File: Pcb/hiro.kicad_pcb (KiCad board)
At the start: 2 copper layers, 80.1 x 107.1 mm, 0 parts

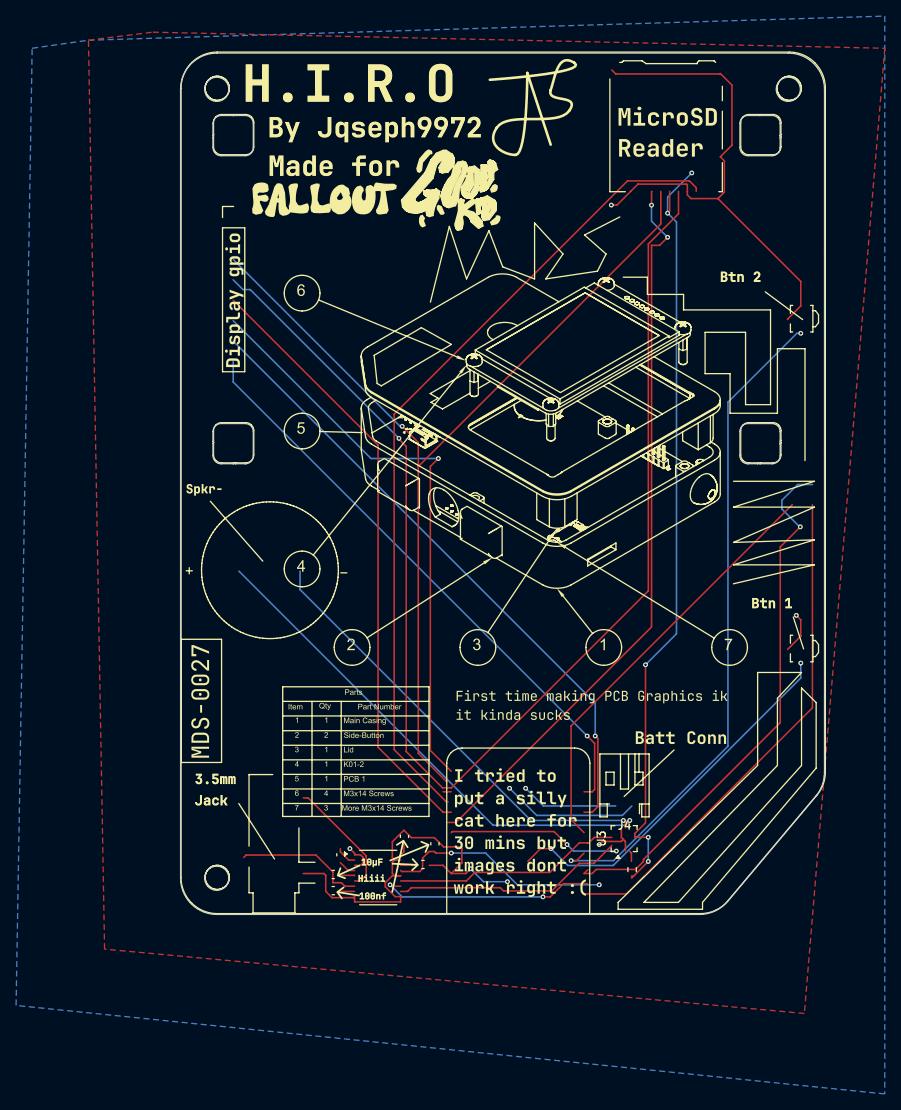
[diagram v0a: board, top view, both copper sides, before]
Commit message: Uh final stuffs i bought emm yayyyy
idk how that pic got there i was sending to my friend idk
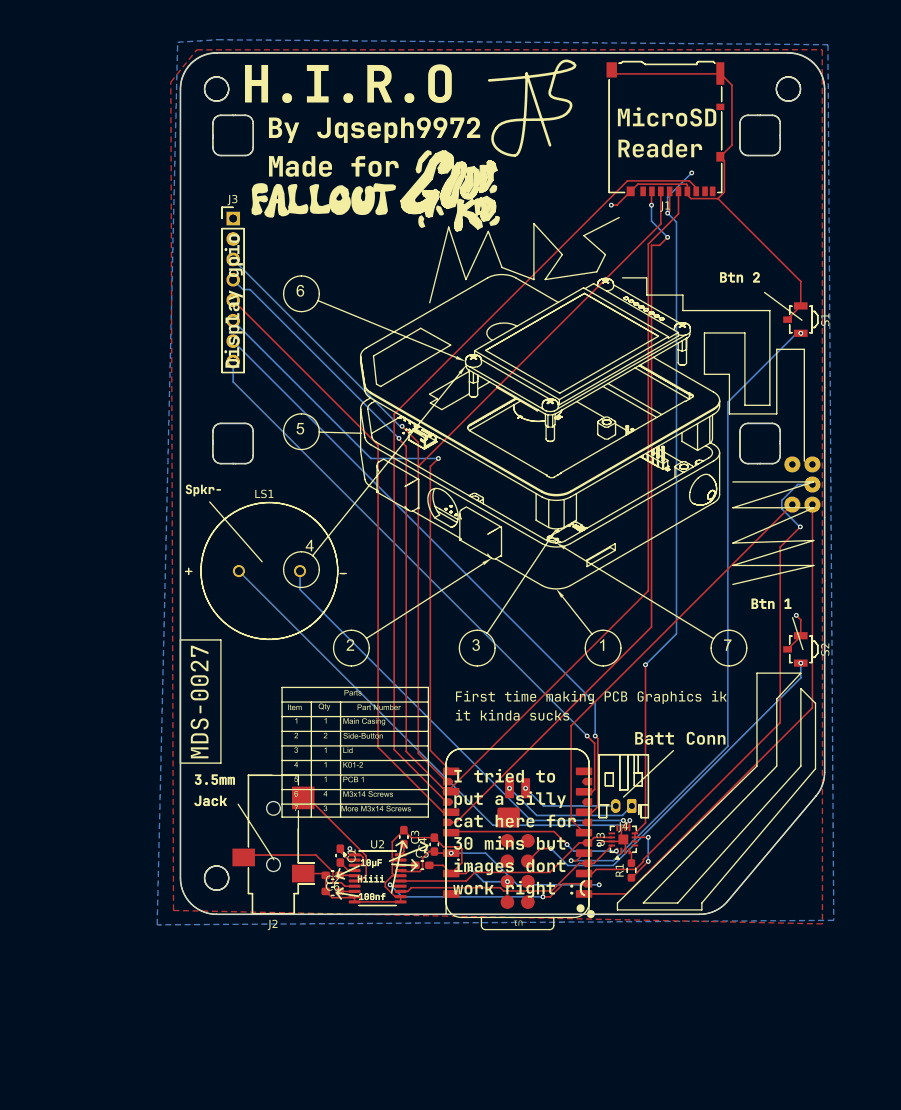
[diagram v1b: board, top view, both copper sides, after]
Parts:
- added C1: 10 µF, Capacitor_SMD:C_0603_1608Metric_Pad1.08x0.95mm_HandSolder, F.Cu at (110.3, 135.4)
- added C2: 100nF, Capacitor_SMD:C_0603_1608Metric_Pad1.08x0.95mm_HandSolder, F.Cu at (109.4, 139.8)
- added C3: 100nF, Capacitor_SMD:C_0603_1608Metric_Pad1.08x0.95mm_HandSolder, F.Cu at (118.2, 133.1)
- added C4: 10 µF, Capacitor_SMD:C_0603_1608Metric_Pad1.08x0.95mm_HandSolder, F.Cu at (122.0, 134.0)
- added C5: 10 µF, Capacitor_SMD:C_0603_1608Metric_Pad1.08x0.95mm_HandSolder, F.Cu at (120.5, 136.6)
- added C6: 10 µF, Capacitor_SMD:C_0603_1608Metric_Pad1.08x0.95mm_HandSolder, F.Cu at (109.4, 137.8)
- added J1: Micro_SD_Card_Det_Hirose_DM3AT, Connector_Card:microSD_HC_Hirose_DM3AT-SF-PEJM5, F.Cu at (150.7, 45.1)
- added J2: AudioJack3, Connector_Audio:Jack_3.5mm_CUI_SJ-3523-SMT_Horizontal, F.Cu at (102.0, 134.0)
- added J3: Conn_01x08, Connector_PinHeader_2.54mm:PinHeader_1x08_P2.54mm_Vertical, F.Cu at (97.0, 56.2)
- added J4: Conn_01x02, Connector_JST:JST_PH_S2B-PH-K_1x02_P2.00mm_Horizontal, F.Cu at (146.6, 129.2)
- added LS1: CVS-1708, Spkr:SPKR_CVS-1708, F.Cu at (101.5, 100.0)
- added R1: 1M, Resistor_SMD:R_0603_1608Metric_Pad0.98x0.95mm_HandSolder, F.Cu at (146.5, 137.2)
- added S1: B3U-3100P-B, Button_Switch_SMD:SW_SPST_B3U-3100P, F.Cu at (166.7, 68.7)
- added S2: B3U-3100P-B, Button_Switch_SMD:SW_SPST_B3U-3100P, F.Cu at (166.7, 109.7)
- added SW1: RotaryEncoder_Switch, Libs:Right angle EC11 Rotary Encoder, F.Cu at (169.0, 91.7)
- added U1: XIAO-ESP32-S3-Plus-SMD, New_XIAO_Series_Footprints:XIAO-ESP32-S3-Plus-SMD, F.Cu at (132.4, 132.5)
- added U2: PCM5102A, Package_SO:TSSOP-20_4.4x6.5mm_P0.65mm, F.Cu at (115.0, 138.2)
- added U3: MAX98357A, Package_DFN_QFN:TQFN-16-1EP_3x3mm_P0.5mm_EP1.23x1.23mm, F.Cu at (145.5, 133.4)
